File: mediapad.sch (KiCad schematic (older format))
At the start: 47 parts, among them SW1 SW_Push, SW2 Rotary_Encoder_Switch, U1 ATmega32U4-AU, Y1 16MHz

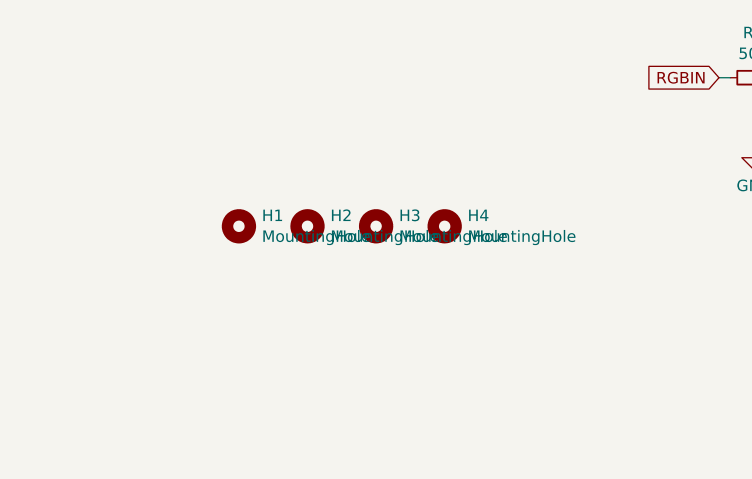
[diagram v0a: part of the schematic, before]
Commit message: updated final pcb design
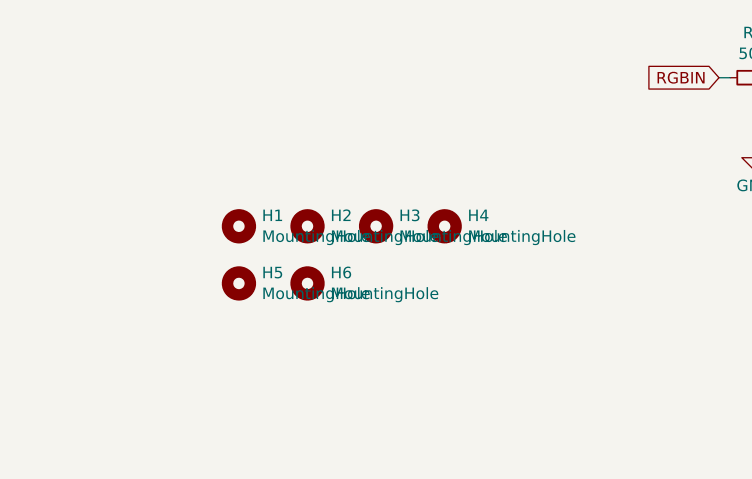
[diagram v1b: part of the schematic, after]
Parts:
- added H5, H6: MountingHole, MountingHole:MountingHole_2.2mm_M2, symbol Mechanical:MountingHole
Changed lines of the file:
@@
 Text GLabel 3500 4200 2    50   Input ~ 0
 COL3
+$Comp
+L Mechanical:MountingHole H5
+U 1 1 5FCCB6B1
+P 1500 6650
+F 0 "H5" H 1600 6696 50  0000 L CNN
+F 1 "MountingHole" H 1600 6605 50  0000 L CNN
+F 2 "MountingHole:MountingHole_2.2mm_M2" H 1500 6650 50  0001 C CNN
+F 3 "~" H 1500 6650 50  0001 C CNN
+	1    1500 6650
+	1    0    0    -1
+$EndComp
+$Comp
+L Mechanical:MountingHole H6
+U 1 1 5FCCBE09
+P 1800 6650
+F 0 "H6" H 1900 6696 50  0000 L CNN
+F 1 "MountingHole" H 1900 6605 50  0000 L CNN
+F 2 "MountingHole:MountingHole_2.2mm_M2" H 1800 6650 50  0001 C CNN
+F 3 "~" H 1800 6650 50  0001 C CNN
+	1    1800 6650
+	1    0    0    -1
+$EndComp
 $EndSCHEMATC
